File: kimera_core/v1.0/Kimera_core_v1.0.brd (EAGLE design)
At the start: 26 x 12 mm, 15 parts, among them IC1 PCA9555RGER, IC2 PCA9555RGER, Q1 CSTCR6M00G53Z, U1 ATMEGA32U4QFN

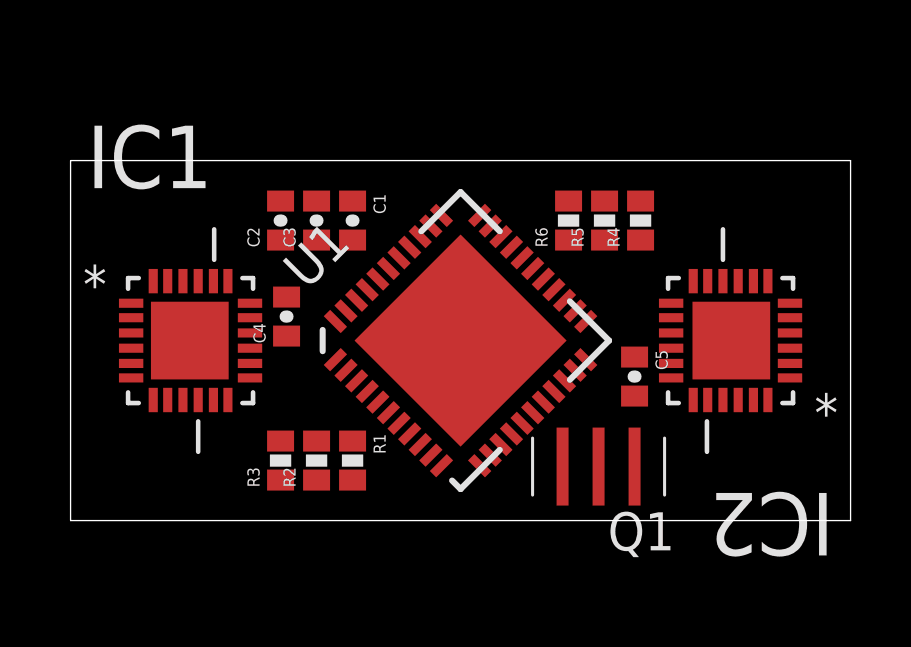
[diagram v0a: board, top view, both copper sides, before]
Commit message: kimera_core: Change bus and layout
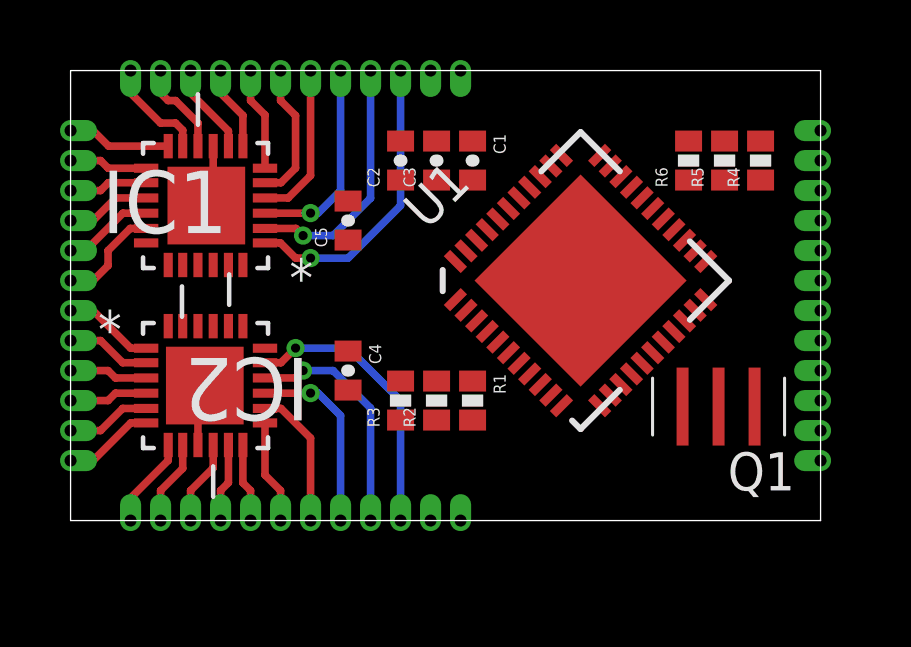
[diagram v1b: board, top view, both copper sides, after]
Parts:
- added JP1, JP2, JP3, JP4: (no value), castellation:P12
- moved IC2 18.1 mm to (4.50, 10.5)
- moved C5 10.9 mm to (9.25, 10.0), turned to 90 degrees
- moved C1 4.47 mm to (13.4, 12.0)
- moved C2 4.47 mm to (11.0, 12.0)
- moved C3 4.47 mm to (12.2, 12.0)
- moved Q1 4.47 mm to (21.6, 3.80)
- moved R1 4.47 mm to (13.4, 4.00)
- moved R2 4.47 mm to (12.2, 4.00)
- moved R3 4.47 mm to (11.0, 4.00)
- moved R4 4.47 mm to (23.0, 12.0)
- moved R5 4.47 mm to (21.8, 12.0)
- moved R6 4.47 mm to (20.6, 12.0)
- moved U1 4.47 mm to (17.0, 8.00)
- moved C4 2.73 mm to (9.25, 5.00), turned to 270 degrees
- moved IC1 1.58 mm to (4.50, 4.50)
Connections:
- net N$1 renamed RESET
- net N$11 renamed SDA
- removed net N$10: IC1.19, R5.1, U1.18
- new net A1: IC1.23, IC2.23
- new net A2: IC1.24, IC2.24
- new net MISO: U1.11
- new net MOSI: U1.10
- new net P1: IC1.1, JP2.7
- new net P10: IC1.11, JP1.4
- new net P11: IC1.12, JP1.5
- new net P12: IC1.13, JP1.6
- new net P13: IC1.14, JP1.7
- new net P14: IC1.15, JP1.8
- new net P15: IC1.16, JP1.9
- new net P16: IC1.17, JP1.10
- new net P17: IC2.1, JP3.3
- new net P18: IC2.2, JP3.4
- new net P19: IC2.3, JP3.5
- new net P2: IC1.2, JP2.8
- new net P20: IC2.4, JP3.6
- new net P21: IC2.5, JP3.7
- new net P22: IC2.6, JP3.8
- new net P23: IC2.7, JP3.9
- new net P24: IC2.8, JP3.10
- new net P25: IC2.10, JP3.11
- new net P26: IC2.11, JP3.12
- new net P27: IC2.12, JP2.1
- new net P28: IC2.13, JP2.2
- new net P29: IC2.14, JP2.3
- new net P3: IC1.3, JP2.9
- new net P30: IC2.15, JP2.4
- new net P31: IC2.16, JP2.5
- new net P32: IC2.17, JP2.6
- new net P4: IC1.4, JP2.10
- new net P5: IC1.5, JP2.11
- new net P6: IC1.6, JP2.12
- new net P7: IC1.7, JP1.1
- new net P8: IC1.8, JP1.2
- new net P9: IC1.10, JP1.3
- new net RX: U1.20
- new net SCK: U1.9
- new net SCL: IC1.19, IC2.19, R5.1, U1.18
- new net TX: U1.21
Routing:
- net P17: track 0.00 -> 9.95 mm, vias 0 -> 1
- net P16: track 0.00 -> 9.45 mm, vias 0 -> 1
- net P18: track 0.00 -> 8.39 mm, vias 0 -> 1
- net P15: track 0.00 -> 7.89 mm, vias 0 -> 1
- net P19: track 0.00 -> 6.83 mm, vias 0 -> 1
- net P14: track 0.00 -> 6.33 mm, vias 0 -> 1
- net P20: track 0.00 -> 5.33 mm
- net P21: track 0.00 -> 4.68 mm
- net P13: track 0.00 -> 4.68 mm
- net GND: track 0.00 -> 4.15 mm
- net P26: track 0.00 -> 3.53 mm
- net P32: track 0.00 -> 3.53 mm
- net P27: track 0.00 -> 3.47 mm
- net P12: track 0.00 -> 3.47 mm
- net P22: track 0.00 -> 3.45 mm
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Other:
- board size 26 x 12 mm -> 25 x 15 mm
